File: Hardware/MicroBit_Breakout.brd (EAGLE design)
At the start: 58.4 x 12.7 mm, 3 parts, among them J1 M22LOCK, X1 EDGE-80PTH-RA

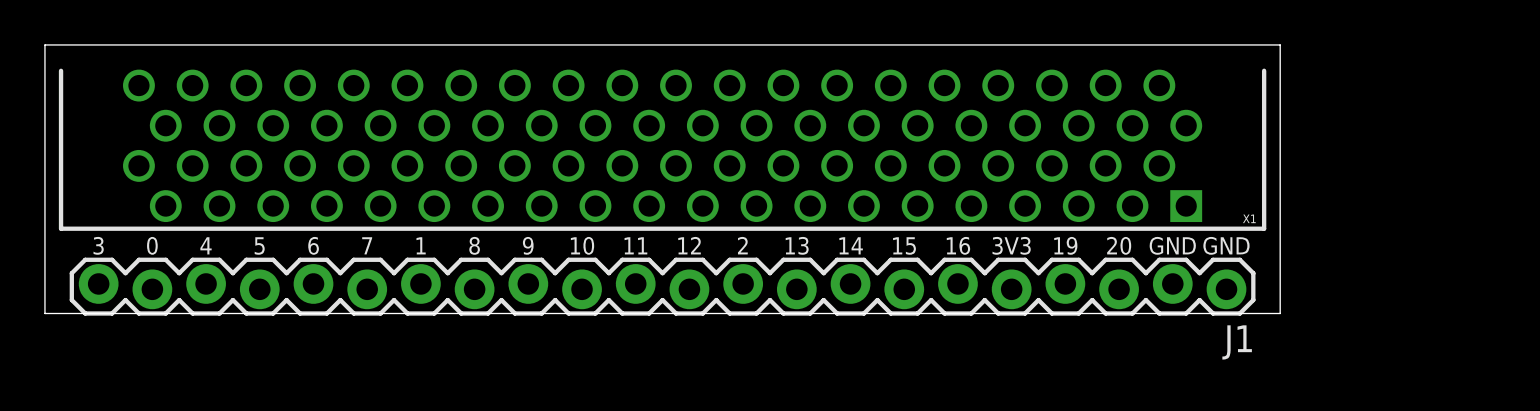
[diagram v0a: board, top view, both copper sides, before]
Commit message: Layout complete
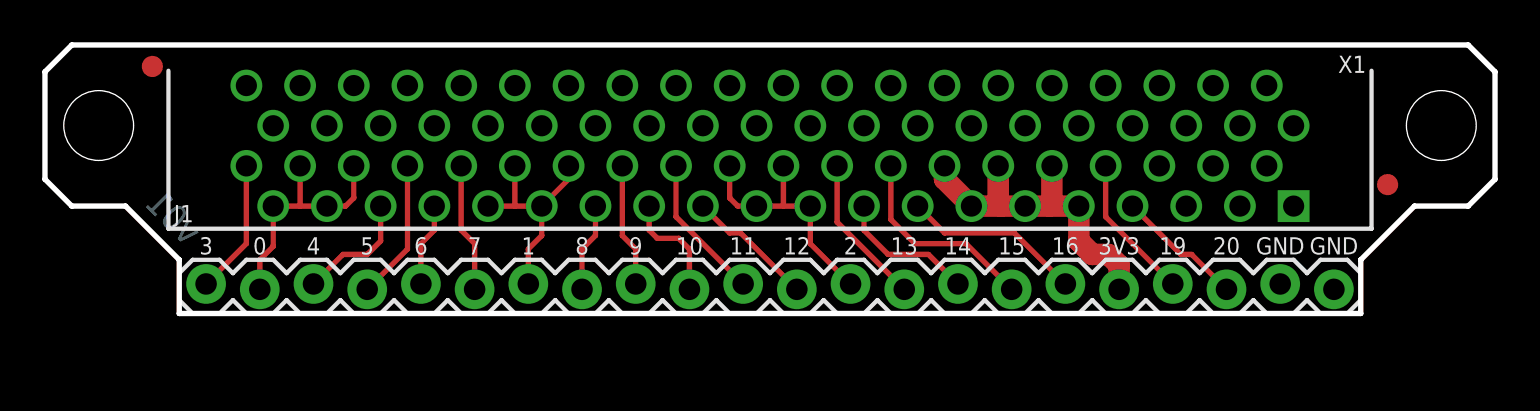
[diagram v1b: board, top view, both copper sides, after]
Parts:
- added FD1, FD2: FIDUCIAL1X2, SparkFun-Aesthetics:FIDUCIAL-1X2
- added H1, H2: STAND-OFF, SparkFun-Electromechanical:STAND-OFF
- added LOGO1: SFE_LOGO_FLAME.1_INCH, SparkFun-Aesthetics:SFE_LOGO_FLAME_.1
- added LOGO3: OSHW-LOGOS, SparkFun-Aesthetics:OSHW-LOGO-S
- moved FRAME1 7.62 mm to (10.2, -11.4)
- moved J1 5.08 mm to (61.0, 1.27)
- moved X1 5.08 mm to (34.3, 5.08)
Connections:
- net N$1 renamed GND
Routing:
- net N$5: track 0.00 -> 16.6 mm
- net N$9: track 0.00 -> 11.9 mm
- net N$21: track 0.00 -> 11.6 mm
- net N$15: track 0.00 -> 10.8 mm
- net N$6: track 0.00 -> 9.62 mm
- net N$2: track 0.00 -> 8.51 mm
- net N$8: track 0.00 -> 7.15 mm
- net N$4: track 0.00 -> 6.90 mm
- net N$11: track 0.00 -> 6.90 mm
- net N$7: track 0.00 -> 6.64 mm
- net N$19: track 0.00 -> 6.63 mm
- net N$22: track 0.00 -> 6.37 mm
- net N$17: track 0.00 -> 6.10 mm
- net N$10: track 0.00 -> 6.08 mm
- net N$3: track 0.00 -> 6.08 mm
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- added copper zone on layer 1, net GND
- added copper zone on layer 16, net GND
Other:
- board size 58.4 x 12.7 mm -> 68.6 x 12.7 mm
- board text added: "Micro Bit Breakout"
- board text added: "Shawn Hymel"
- board text added: "v01"
